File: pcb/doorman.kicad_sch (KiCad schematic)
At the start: 56 parts, among them J1 USB-C Connector, J2 Screw Terminals, J3 3V3 Test Pad, J4 Extension Board Connector, J6 BUS Test Pad, J7 BUS RX Test Pad, J8 TX Test Pad, J9 RX Test Pad, Q1 BC847BPN, Q2 BC817-40, Q3 BC817-40, Q4 BC817-40, Q5 BC807-40, Q6 BC807-40, SW1 Button, SW2 Button, U2 AP63203WU, U3 GAQY252G3S, U4 ESP32-S3-MINI-1

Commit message: WIP
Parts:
- J1: Cheap Version C2765186 -> (none); Expensive Version C165948 -> (none); LCSC C2765186 -> C165948; MPN TYPE-C 16PIN 2MD(073) -> TYPE-C-31-M-12
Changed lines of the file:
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@@
 			)
 		)
-		(property "Description" "5A 1 Surface Mount，Right Angle 16P Female -25℃~+85℃ Type-C SMD USB Connectors ROHS"
+		(property "Description" "-30℃~+80℃ 1 10,000 cycles 16P 20V 5A 7.35mm Female Surface Mount, Right Angle Type-C SMD USB Connectors ROHS"
 			(at 242.57 85.09 0)
 			(effects
@@
 			)
 		)
-		(property "LCSC" "C2765186"
+		(property "LCSC" "C165948"
 			(at 242.57 85.09 90)
 			(effects
@@
 			)
 		)
-		(property "MPN" "TYPE-C 16PIN 2MD(073)"
-			(at 242.57 85.09 0)
-			(effects
-				(font
-					(size 1.27 1.27)
-				)
-				(hide yes)
-			)
-		)
-		(property "Cheap Version" "C2765186"
-			(at 242.57 85.09 0)
-			(effects
-				(font
-					(size 1.27 1.27)
-				)
-				(hide yes)
-			)
-		)
-		(property "Expensive Version" "C165948"
-			(at 242.57 85.09 0)
-			(effects
-				(font
-					(size 1.27 1.27)
-				)
-				(hide yes)
-			)
-		)
-		(property "Price" ""
+		(property "MPN" "TYPE-C-31-M-12"
 			(at 242.57 85.09 0)
 			(effects
@@
 			(at 242.57 85.09 0)
 			(effects
-				(font
-					(size 1.27 1.27)
-				)
-				(hide yes)
-			)
-		)
-		(property "Manufacturer_Name" ""
-			(at 242.57 85.09 0)
-			(effects
-				(font
-					(size 1.27 1.27)
-				)
-				(hide yes)
-			)
-		)
-		(property "Manufacturer_Part_Number" ""
-			(at 242.57 85.09 0)
-			(effects

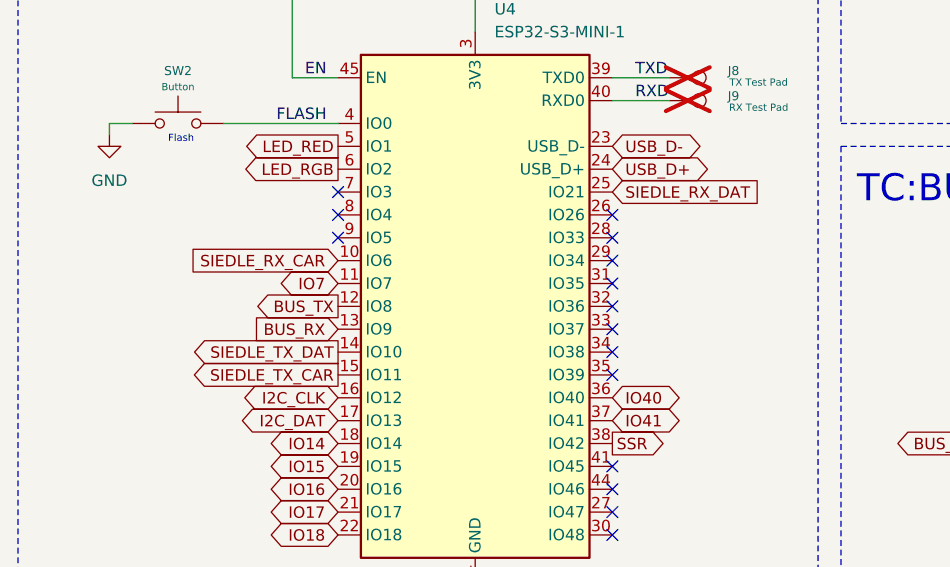
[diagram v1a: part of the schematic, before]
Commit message: WIP
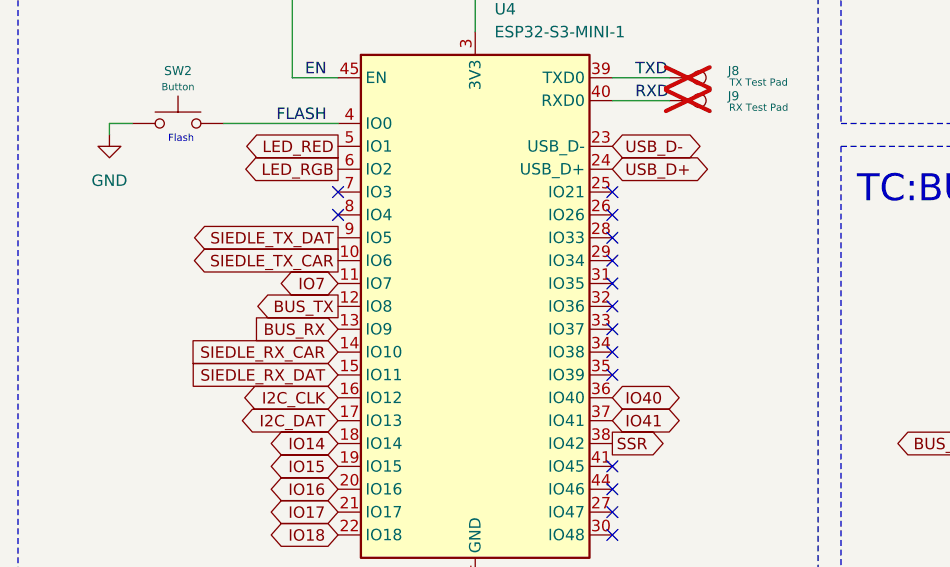
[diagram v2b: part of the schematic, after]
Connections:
- net SIEDLE_RX_CAR: now also U4.14 (IO10); no longer U4.10 (IO6)
- net SIEDLE_RX_DAT: now also U4.15 (IO11); no longer U4.25 (IO21)
- net SIEDLE_TX_CAR: now also U4.10 (IO6); no longer U4.15 (IO11)
- net SIEDLE_TX_DAT: now also U4.9 (IO5); no longer U4.14 (IO10)
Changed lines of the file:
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@@
 	(title_block
 		(title "Doorman S3")
-		(date "2026-02-16")
+		(date "2026-02-17")
 		(rev "2.0")
 		(comment 1 "TC:Bus Intercom Gateway")
@@
 	)
 	(no_connect
-		(at 52.07 81.28)
-	)
-	(no_connect
 		(at 82.55 106.68)
 	)
@@
 	)
 	(no_connect
+		(at 82.55 76.2)
+	)
+	(no_connect
 		(at 82.55 96.52)
 	)
@@
 		)
 	)
+	(global_label "SIEDLE_TX_DAT"
+		(shape output)
+		(at 52.07 81.28 180)
+		(fields_autoplaced yes)
+		(effects
+			(font
+				(size 1.27 1.27)
+			)
+			(justify right)
+		)
+		(property "Intersheetrefs" "${INTERSHEET_REFS}"
+			(at 41.8277 81.28 0)
+			(effects
+				(font
+					(size 1.27 1.27)
+				)
+				(justify right)
+				(hide yes)
+			)
+		)
+	)
 	(global_label "BUS_RX"
 		(shape input)
@@
 		)
 	)
+	(global_label "SIEDLE_TX_CAR"
+		(shape output)
+		(at 52.07 83.82 180)
+		(fields_autoplaced yes)
+		(effects
+			(font
+				(size 1.27 1.27)
+			)
+			(justify right)
+		)
+		(property "Intersheetrefs" "${INTERSHEET_REFS}"
+			(at 41.8277 83.82 0)
+			(effects
+				(font
+					(size 1.27 1.27)
+				)
+				(justify right)
+				(hide yes)
+			)
+		)
+	)
 	(global_label "BUS_TX"
 		(shape output)
@@
 	(global_label "SIEDLE_RX_DAT"
 		(shape input)
-		(at 82.55 76.2 0)
+		(at 52.07 96.52 180)
 		(fields_autoplaced yes)
 		(effects
@@
 				(size 1.27 1.27)
 			)
-			(justify left)
+			(justify right)
 		)
 		(property "Intersheetrefs" "${INTERSHEET_REFS}"
-			(at 99.6865 76.2 0)
+			(at 34.9335 96.52 0)
 			(effects
 				(font
 					(size 1.27 1.27)
 				)
-				(justify left)
+				(justify right)
+				(hide yes)
+			)
+		)
+	)
+	(global_label "SIEDLE_RX_CAR"
+		(shape input)
+		(at 52.07 93.98 180)
+		(fields_autoplaced yes)
+		(effects
+			(font
+				(size 1.27 1.27)
+			)
+			(justify right)
+		)
+		(property "Intersheetrefs" "${INTERSHEET_REFS}"
+			(at 33.7844 93.98 0)
+			(effects
+				(font
+					(size 1.27 1.27)
+				)
+				(justify right)
 				(hide yes)
 			)
@@
 		)
 	)
-	(global_label "SIEDLE_TX_CAR"
-		(shape output)
-		(at 52.07 96.52 180)
-		(fields_autoplaced yes)
-		(effects
-			(font
-				(size 1.27 1.27)
-			)
-			(justify right)
-		)
-		(property "Intersheetrefs" "${INTERSHEET_REFS}"
-			(at 41.8277 96.52 0)
-			(effects
-				(font
-					(size 1.27 1.27)
-				)
-				(justify right)
-				(hide yes)
-			)
-		)
-	)
 	(global_label "I2C_DAT"
 		(shape bidirectional)
@@
 		)
 	)
-	(global_label "SIEDLE_TX_DAT"
-		(shape output)
-		(at 52.07 93.98 180)
-		(fields_autoplaced yes)
-		(effects
-			(font
-				(size 1.27 1.27)
-			)
-			(justify right)
-		)
-		(property "Intersheetrefs" "${INTERSHEET_REFS}"
-			(at 41.8277 93.98 0)
-			(effects
-				(font
-					(size 1.27 1.27)
-				)
-				(justify right)
-				(hide yes)
-			)
-		)
-	)
 	(global_label "SIEDLE_TX_CAR"
 		(shape output)
@@
 				(hide yes)
 			)
-		)
-	)
-	(global_label "SIEDLE_RX_CAR"
-		(shape input)
-		(at 52.07 83.82 180)
-		(fields_autoplaced yes)
-		(effects
-			(font
-				(size 1.27 1.27)
-			)
-			(justify right)
-		)
-		(property "Intersheetrefs" "${INTERSHEET_REFS}"
-			(at 33.7844 83.82 0)
-			(effects
-				(font
-					(size 1.27 1.27)
-				)
-				(justify right)
-				(hide yes)
-			)

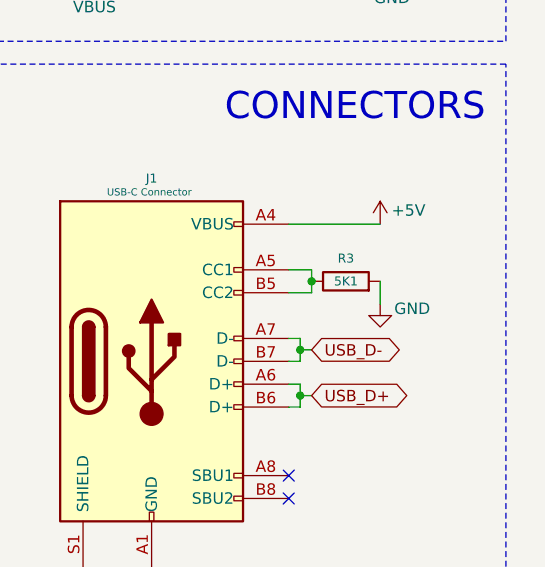
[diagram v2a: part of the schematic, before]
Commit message: WIP
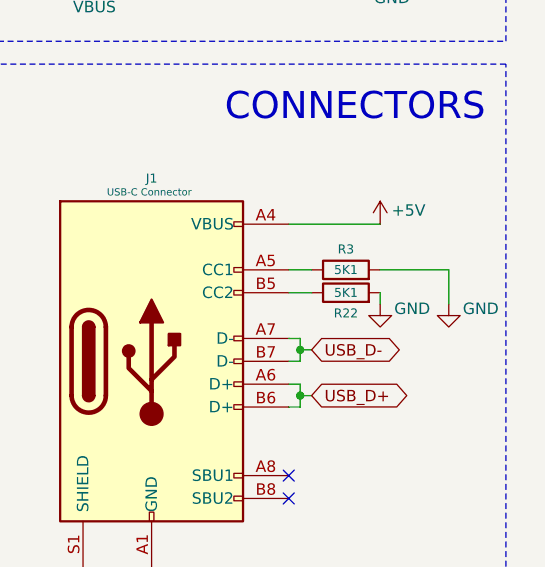
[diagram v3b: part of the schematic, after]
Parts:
- added R22: 5K1, Resistor_SMD:R_0402_1005Metric, symbol Device:R
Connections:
- net GND: now also R22.2
- net at J1.B5 (CC2), R3.1: no longer J1.A5 (CC1)
- new net: J1.A5 (CC1), R22.1
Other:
- moved on the sheet: R3

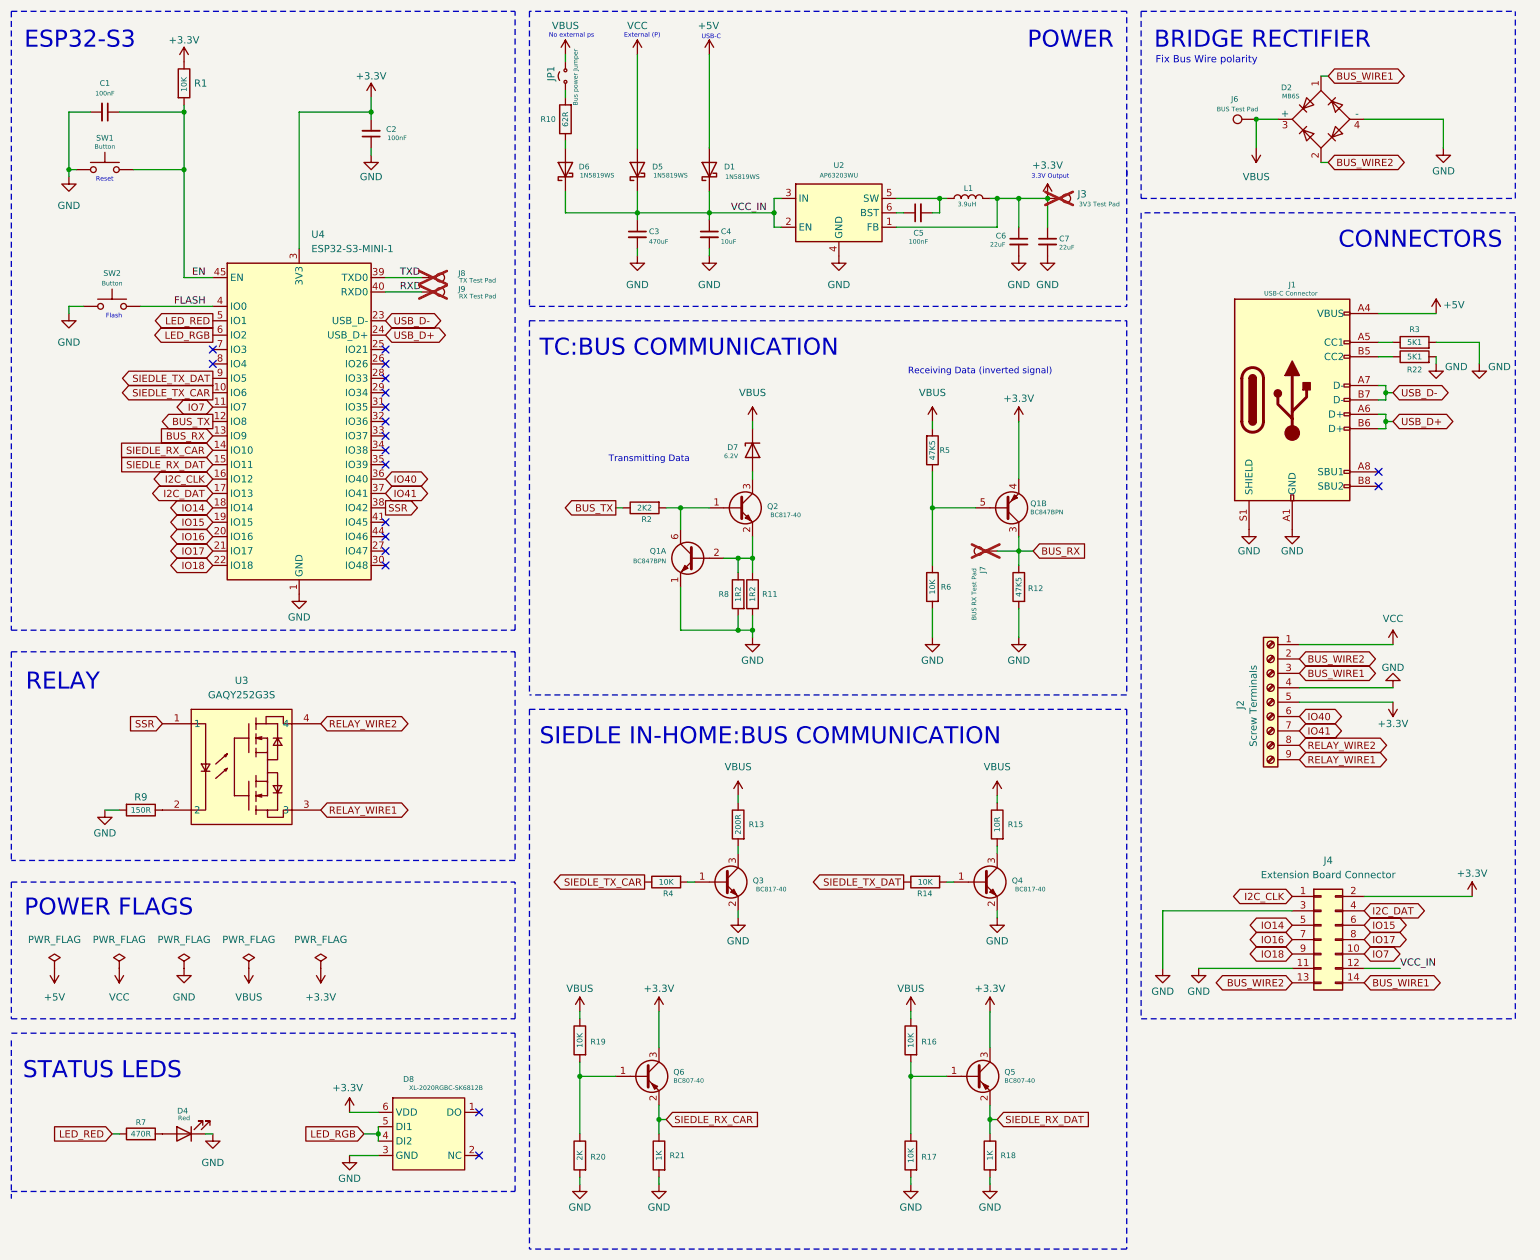
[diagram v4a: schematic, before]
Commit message: WIP
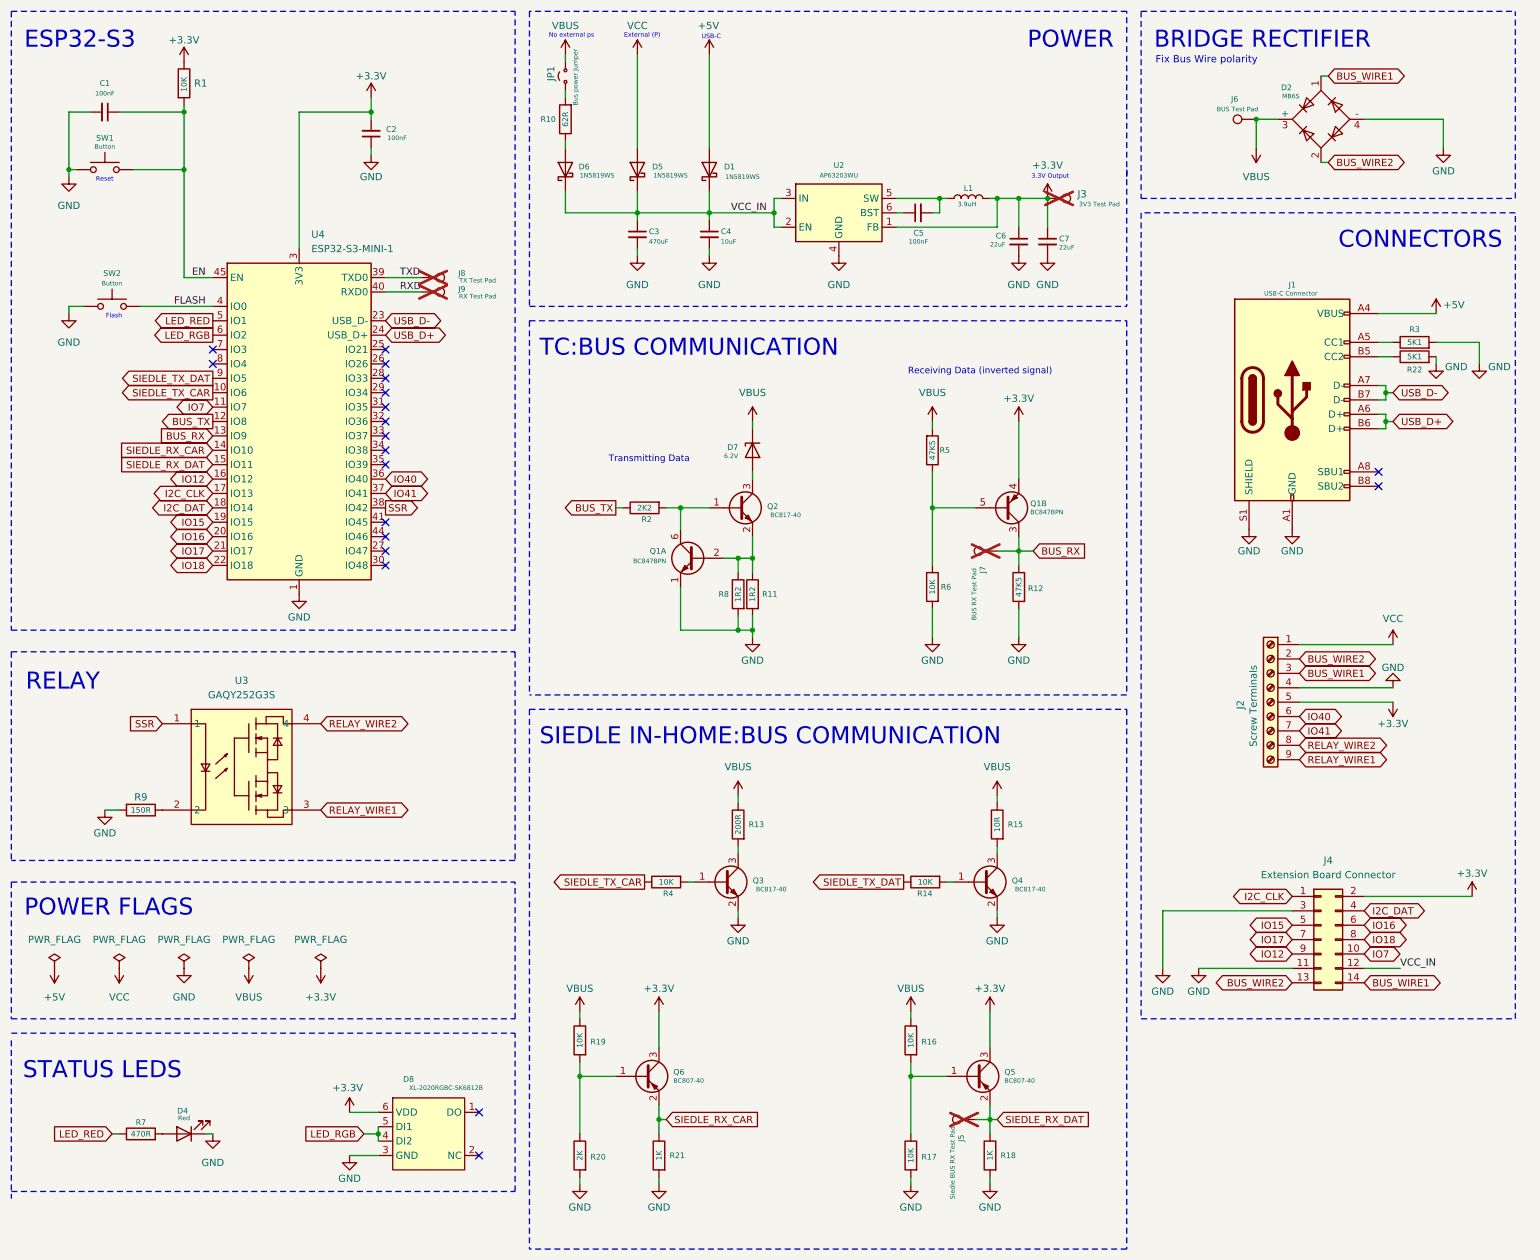
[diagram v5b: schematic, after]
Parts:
- added J5: Siedle BUS RX Test Pad, TestPoint:TestPoint_Pad_D1.0mm, symbol Connector:TestPoint
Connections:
- net I2C_CLK: now also U4.17 (IO13); no longer U4.16 (IO12)
- net I2C_DAT: now also U4.18 (IO14); no longer U4.17 (IO13)
- net IO15: now also J4.5 (Pin_5); no longer J4.6 (Pin_6)
- net IO16: now also J4.6 (Pin_6); no longer J4.7 (Pin_7)
- net IO17: now also J4.7 (Pin_7); no longer J4.8 (Pin_8)
- net IO18: now also J4.8 (Pin_8); no longer J4.9 (Pin_9)
- net SIEDLE_RX_DAT: now also J5.1
- removed net IO14: J4.5 (Pin_5), U4.18 (IO14)
- new net IO12: J4.9 (Pin_9), U4.16 (IO12)

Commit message: WIP
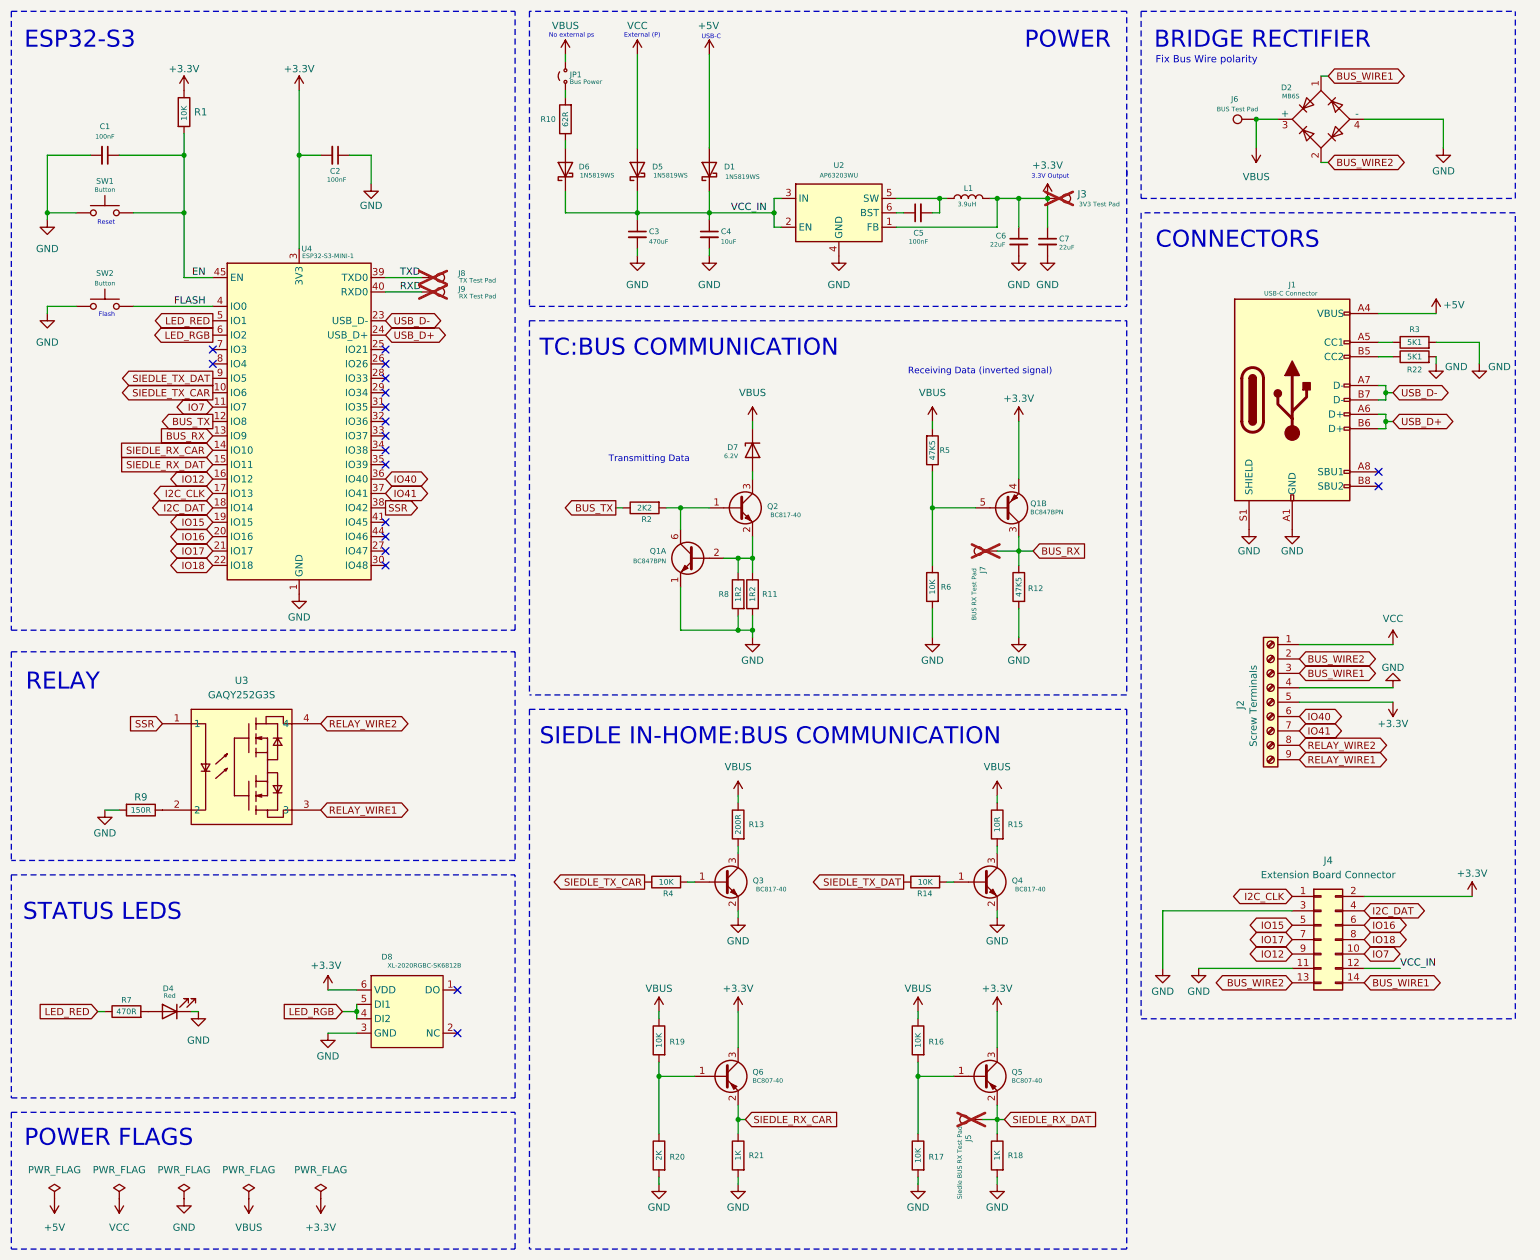
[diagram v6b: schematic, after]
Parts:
- JP1: value Bus power Jumper -> Bus Power
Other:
- moved on the sheet: C1, C2, D4, D8, J5, Q5, Q6, R1, R16, R17, R18, R19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
